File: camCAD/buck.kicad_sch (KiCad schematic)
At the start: 21 parts, among them J1 USB C Charging Port, J3 BATTERY, U1 BQ24072RGTR Charging IC, U2 SC189ZSKTRT

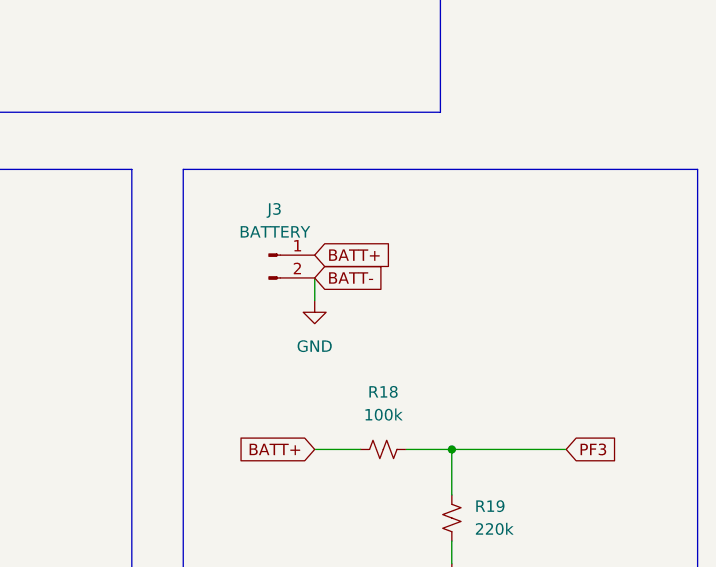
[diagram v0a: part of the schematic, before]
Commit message: layout partially complete
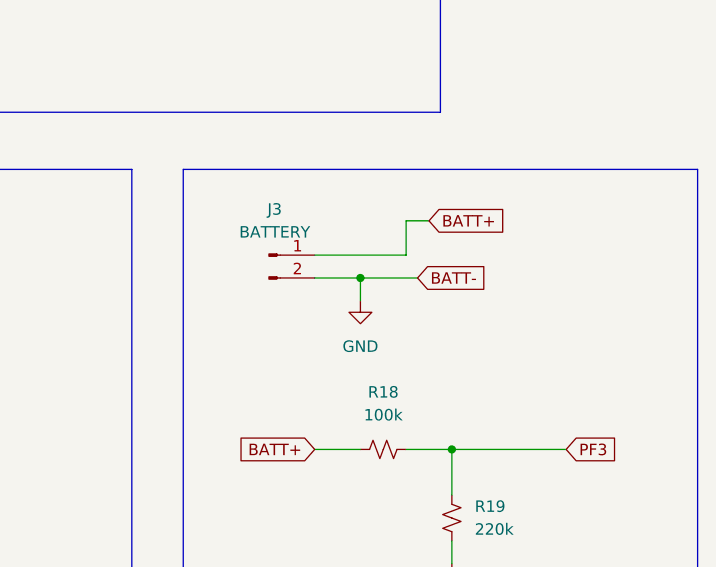
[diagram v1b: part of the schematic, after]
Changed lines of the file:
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@@
+	)
+	(junction
+		(at 219.71 82.55)
+		(diameter 0)
+		(color 0 0 0 0)
 	)
 	(junction
@@
 	(wire
 		(pts
+			(xy 224.79 80.01) (xy 224.79 76.2)
+		)
+		(stroke
+			(width 0)
+			(type default)
+		)
+	)
+	(wire
+		(pts
+			(xy 214.63 80.01) (xy 224.79 80.01)
+		)
+		(stroke
+			(width 0)
+			(type default)
+		)
+	)
+	(wire
+		(pts
 			(xy 163.83 83.82) (xy 156.21 83.82)
 		)
@@
 	(wire
 		(pts
+			(xy 219.71 82.55) (xy 214.63 82.55)
+		)
+		(stroke
+			(width 0)
+			(type default)
+		)
+	)
+	(wire
+		(pts
 			(xy 140.97 30.48) (xy 144.78 30.48)
 		)
@@
 	(wire
 		(pts
+			(xy 219.71 82.55) (xy 219.71 85.09)
+		)
+		(stroke
+			(width 0)
+			(type default)
+		)
+	)
+	(wire
+		(pts
 			(xy 113.03 101.6) (xy 113.03 105.41)
 		)
@@
 	(wire
 		(pts
+			(xy 224.79 76.2) (xy 227.33 76.2)
+		)
+		(stroke
+			(width 0)
+			(type default)
+		)
+	)
+	(wire
+		(pts
 			(xy 153.67 38.1) (xy 153.67 33.02)
 		)
@@
 	(wire
 		(pts
-			(xy 214.63 82.55) (xy 214.63 85.09)
-		)
-		(stroke
-			(width 0)
-			(type default)
-		)
-	)
-	(wire
-		(pts
 			(xy 175.26 106.68) (xy 175.26 114.3)
 		)
@@
 		(pts
 			(xy 175.26 121.92) (xy 175.26 124.46)
+		)
+		(stroke
+			(width 0)
+			(type default)
+		)
+	)
+	(wire
+		(pts
+			(xy 219.71 82.55) (xy 226.06 82.55)
 		)
 		(stroke
@@
 	(global_label "BATT+"
 		(shape input)
-		(at 214.63 80.01 0)
+		(at 227.33 76.2 0)
 		(fields_autoplaced yes)
 		(effects
@@
 		)
 		(property "Intersheetrefs" "${INTERSHEET_REFS}"
-			(at 223.4814 80.01 0)
+			(at 236.1814 76.2 0)
 			(hide yes)
 			(show_name no)
@@
 	(global_label "BATT-"
 		(shape input)
-		(at 214.63 82.55 0)
+		(at 226.06 82.55 0)
 		(fields_autoplaced yes)
 		(effects
@@
 		)
 		(property "Intersheetrefs" "${INTERSHEET_REFS}"
-			(at 223.4814 82.55 0)
+			(at 234.9114 82.55 0)
 			(hide yes)
 			(show_name no)
@@
 	(symbol
 		(lib_id "power:GND")
-		(at 214.63 85.09 0)
+		(at 219.71 85.09 0)
 		(unit 1)
 		(body_style 1)
@@
 		(fields_autoplaced yes)
 		(property "Reference" "#PWR017"
-			(at 214.63 91.44 0)
+			(at 219.71 91.44 0)
 			(hide yes)
 			(show_name no)
@@
 		)
 		(property "Value" "GND"
-			(at 214.63 90.17 0)
+			(at 219.71 90.17 0)
 			(show_name no)
 			(do_not_autoplace no)
@@
 		)
 		(property "Footprint" ""
-			(at 214.63 85.09 0)
+			(at 219.71 85.09 0)
 			(hide yes)
 			(show_name no)
@@
 		)
 		(property "Datasheet" ""
-			(at 214.63 85.09 0)
+			(at 219.71 85.09 0)
 			(hide yes)
 			(show_name no)
@@
 		)
 		(property "Description" "Power symbol creates a global label with name \"GND\" , ground"
-			(at 214.63 85.09 0)
-			(hide yes)
-			(show_name no)
+			(at 219.71 85.09 0)
+			(hide yes)
+			(show_name no)
